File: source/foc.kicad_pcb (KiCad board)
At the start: 4 copper layers, 75.2 x 99.5 mm, 261 parts, among them J1 Conn_01x02_Male, J2 Conn_01x06, J3 communication, J4 on/off, J5 servo, J6 TYPE-C-31-M-12, P1 SWD, P10 SWD, P11 SWD, P12 SWD, P13 SWD, P2 SWD, P3 SWD, P4 SWD, P5 SWD, P6 SWD, P7 SWD, P8 SWD, P9 SWD, Q1 AO3401A, Q10 CRST030N10N, Q11 CRST030N10N, Q12 CRST030N10N, Q13 CRST030N10N, Q14 CRST030N10N, Q15 CRST030N10N, Q16 SS8050, Q2 SS8050, Q3 SS8050, Q4 CRST030N10N, Q5 CRST030N10N, Q6 CRST030N10N, Q7 CRST030N10N, Q8 CRST030N10N, Q9 CRST030N10N, SW1 SW_SPDT, SW2 SW_SPST, SW3 SW_SPST, SW4 SW_SPDT, U1 TJA1051T/3/1J, U10 MS8311, U11 MS8311, U12 STM32F401CCU6_Blackpill, U13 STM32F401CCU6_Blackpill, U14 STM32F405RGT6, U2 BMI270, U3 AMS1117-3.3, U4 IRS21867S, U5 XL1509-5.0E1, U6 IRS21867S, U7 IRS21867S, U8 TX4130L/PW2902, U9 MS8311, Y1 8MHz Crystal Resonator, X5032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

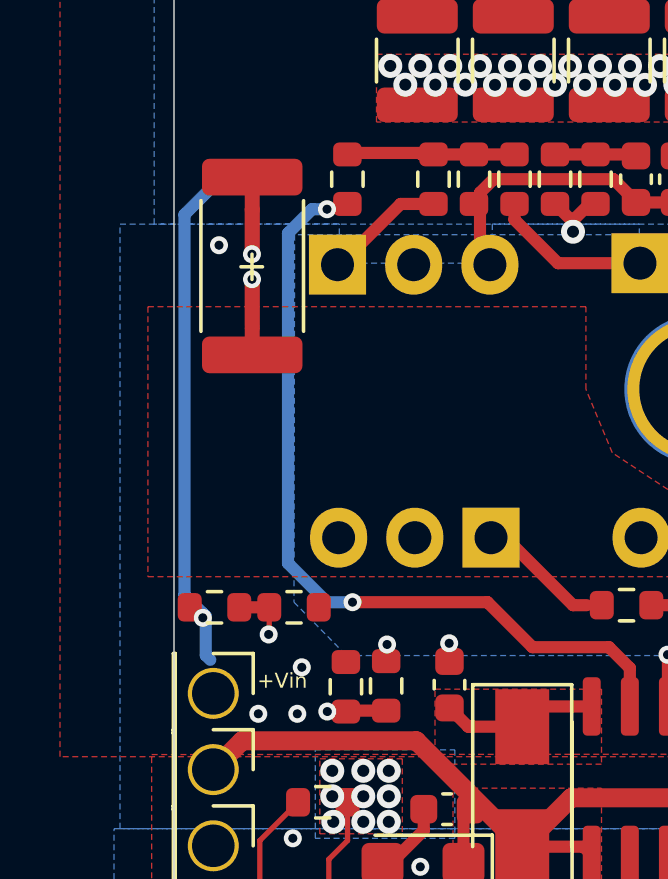
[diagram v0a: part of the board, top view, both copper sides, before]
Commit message: DRC run
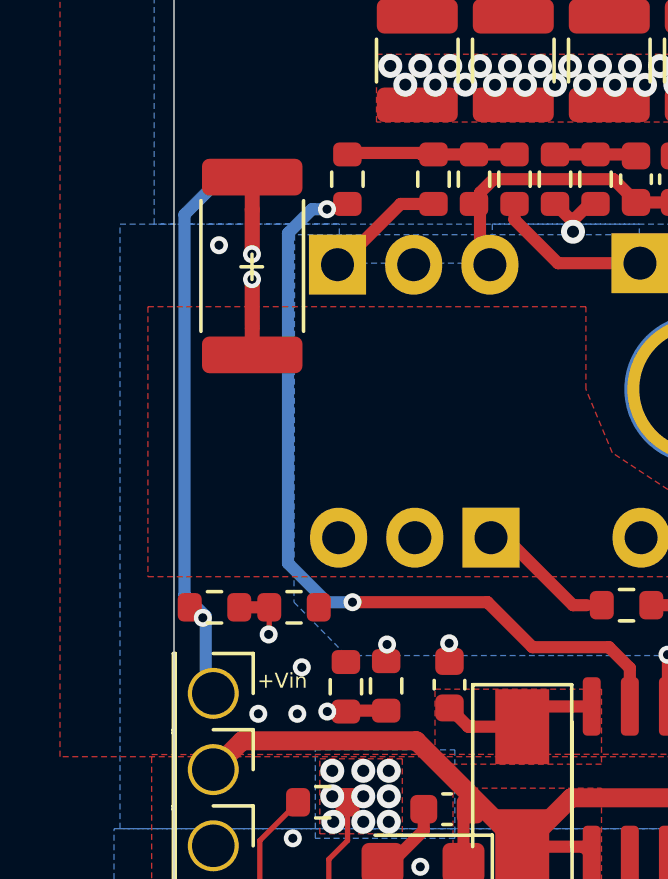
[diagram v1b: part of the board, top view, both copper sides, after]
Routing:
- net V_IN: track 33.4 -> 34.5 mm
- net /driver/SENS_SUPPLY: track 53.0 -> 52.5 mm
- net VCC: vias 17 -> 16
- net GND: vias 406 -> 407
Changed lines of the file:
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@@
 		(tags "capacitor")
 		(property "Reference" "C26"
-			(at 0 -2.3 360)
+			(at 0 -2.3 0)
 			(layer "F.SilkS")
 			(hide yes)
@@
 		)
 		(property "Value" "4.7u 100V"
-			(at 0 2.3 360)
+			(at 0 2.3 0)
 			(layer "F.Fab")
 			(effects
@@
 		)
 		(property "Footprint" "Capacitor_SMD:C_1210_3225Metric"
-			(at 0 0 360)
+			(at 0 0 0)
 			(layer "F.Fab")
 			(hide yes)
@@
 		)
 		(property "Datasheet" ""
-			(at 0 0 360)
+			(at 0 0 0)
 			(layer "F.Fab")
 			(hide yes)
@@
 		)
 		(property "Description" ""
-			(at 0 0 360)
+			(at 0 0 0)
 			(layer "F.Fab")
 			(hide yes)
@@
 		)
 		(property "LCSC" "C381466"
-			(at 390.260002 133.7 360)
+			(at 390.260002 133.7 0)
 			(layer "F.Fab")
 			(hide yes)
@@
 		)
 		(fp_text user "${REFERENCE}"
-			(at 0 0 360)
+			(at 0 0 0)
 			(layer "F.Fab")
 			(effects
@@
 	)
 	(via
-		(at 162.74 125.92)
-		(size 0.6)
-		(drill 0.3)
-		(layers "F.Cu" "B.Cu")
-		(free yes)
-		(net 3)
-	)
-	(via
 		(at 160.33 136.3)
 		(size 0.6)
@@
 	)
 	(segment
-		(start 125.46 91.77)
-		(end 124.85 91.16)
-		(width 0.4064)
-		(layer "B.Cu")
-		(net 7)
-	)
-	(segment
 		(start 124.85 78.48)
-		(end 125.8 77.53)
+		(end 124.85 91.16)
 		(width 0.4064)
 		(layer "B.Cu")
@@
 	)
 	(segment
-		(start 124.85 91.16)
-		(end 124.85 78.48)
+		(start 125.56 91.87)
+		(end 125.56 94.19)
 		(width 0.4064)
 		(layer "B.Cu")
@@
 	)
 	(segment
-		(start 125.56 93.17)
-		(end 125.71 93.32)
+		(start 125.56 94.19)
+		(end 125.81 94.44)
 		(width 0.4064)
 		(layer "B.Cu")
@@
 	)
 	(segment
-		(start 125.46 91.77)
+		(start 124.85 91.16)
 		(end 125.56 91.87)
 		(width 0.4064)
@@
 	)
 	(segment
-		(start 125.56 91.87)
-		(end 125.56 93.17)
+		(start 125.8 77.53)
+		(end 124.85 78.48)
 		(width 0.4064)
 		(layer "B.Cu")
@@
 	)
 	(segment
-		(start 126.675 91.57)
-		(end 127.175411 91.57)
-		(width 0.1778)
-		(layer "F.Cu")
-		(net 27)
-	)
-	(segment
 		(start 143.02 125.41)
 		(end 141.5225 126.9075)
@@
 		(size 0.6)
 		(drill 0.3)
+		(layers "F.Cu" "B.Cu")
+		(free yes)
+		(net 44)
+	)
+	(via
+		(at 162.74 125.92)
+		(size 0.6)
+		(drill 0.3)
